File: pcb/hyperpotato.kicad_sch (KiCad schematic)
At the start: 60 parts, among them J2 Conn_01x02_Socket, J3 Conn_01x04, J4 Conn_01x04, J5 Conn_01x04, J6 Conn_01x12_Socket, J7 Conn_01x12_Socket, K1 SW_Push, K10 SW_Push, K11 SW_Push, K12 SW_Push, K13 SW_Push, K14 SW_Push, K15 SW_Push, K16 SW_Push, K17 SW_Push, K2 SW_Push, K3 SW_Push, K4 SW_Push, K5 SW_Push, K6 SW_Push, K7 SW_Push, K8 SW_Push, K9 SW_Push, SW1 SW_Push, SW2 SW_SPDT, U1 ProMicro

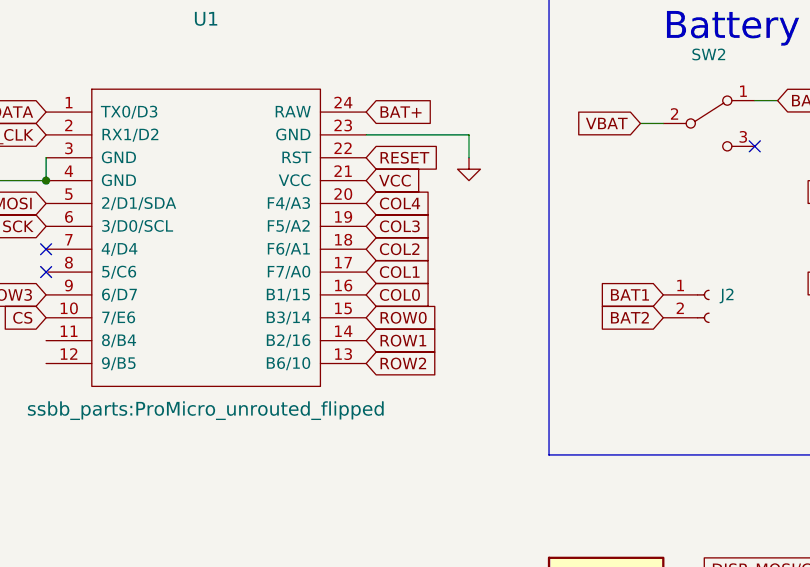
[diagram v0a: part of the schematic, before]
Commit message: Finish v2
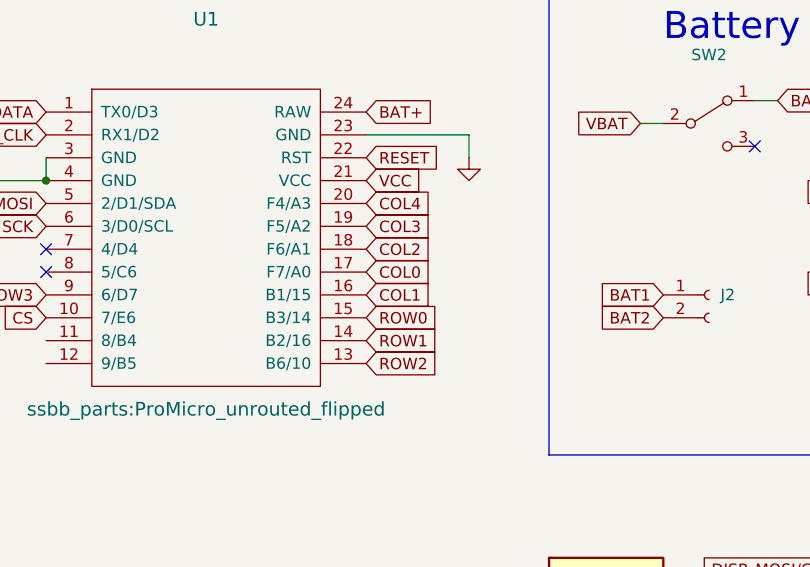
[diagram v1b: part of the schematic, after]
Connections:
- net COL0: now also U1.17 (F7/A0); no longer U1.16 (B1/15)
- net COL1: now also U1.16 (B1/15); no longer U1.17 (F7/A0)
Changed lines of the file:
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@@
     )
   )
-  (global_label "COL0" (shape input) (at 186.69 53.34 0) (fields_autoplaced)
+  (global_label "COL1" (shape input) (at 186.69 53.34 0) (fields_autoplaced)
     (effects (font (size 1.27 1.27)) (justify left))
     (property "Intersheetrefs" "${INTERSHEET_REFS}" (at 194.5133 53.34 0)
@@
     )
   )
-  (global_label "COL1" (shape input) (at 186.69 50.8 0) (fields_autoplaced)
+  (global_label "COL0" (shape input) (at 186.69 50.8 0) (fields_autoplaced)
     (effects (font (size 1.27 1.27)) (justify left))
     (property "Intersheetrefs" "${INTERSHEET_REFS}" (at 194.5133 50.8 0)

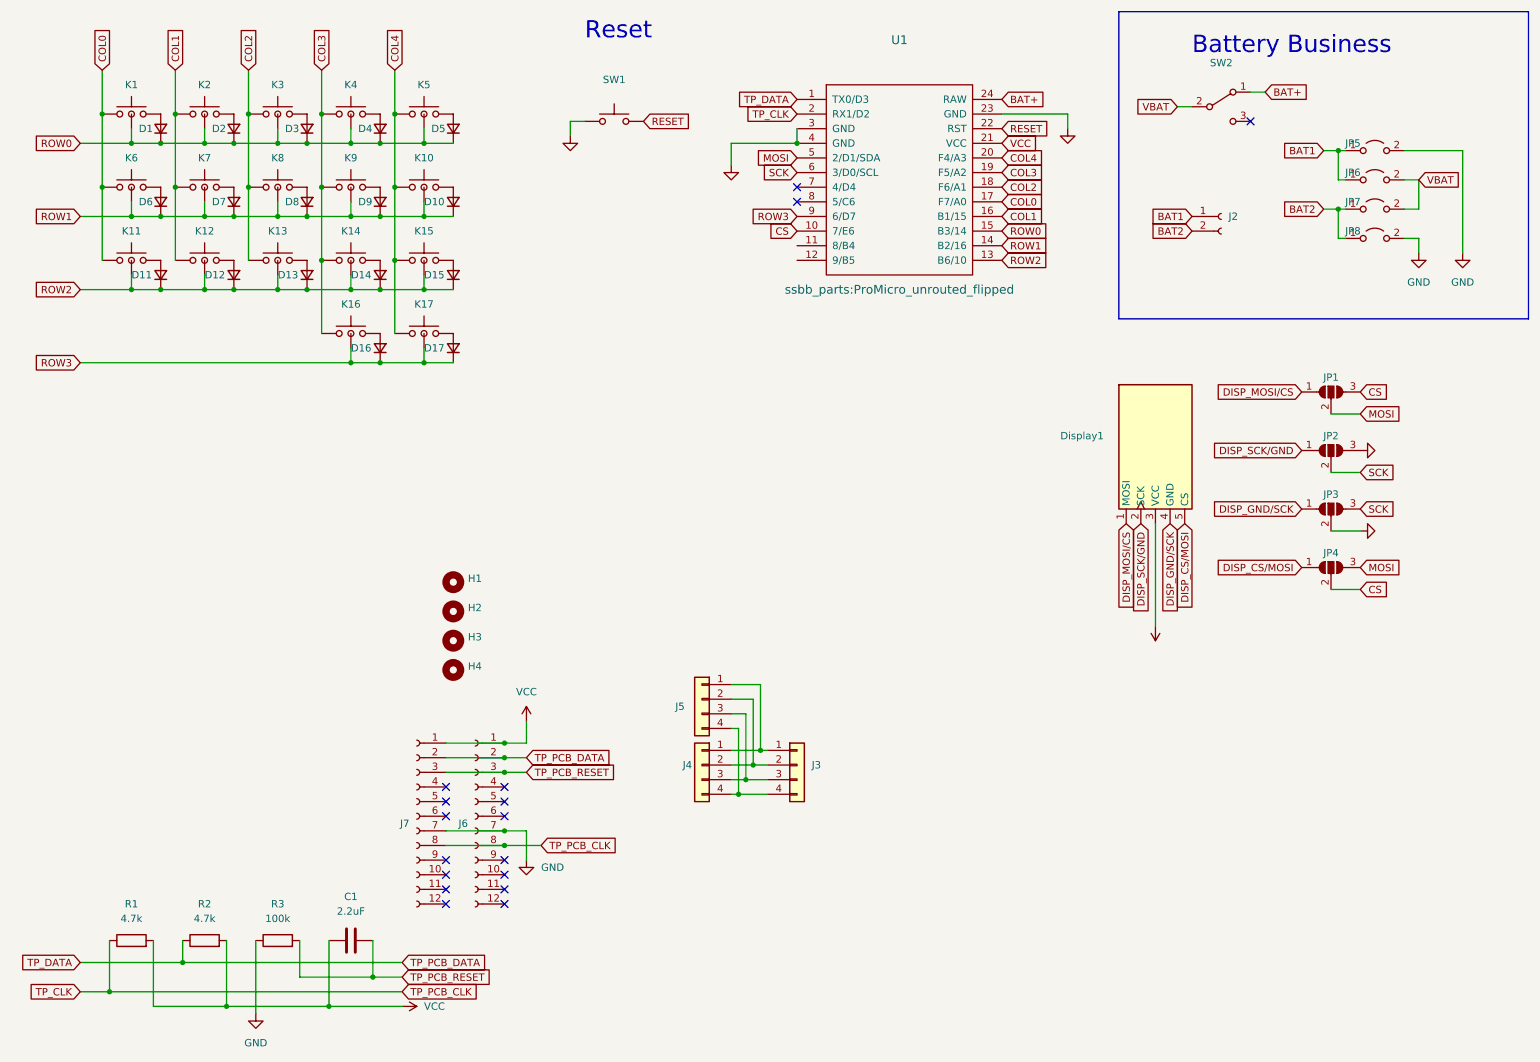
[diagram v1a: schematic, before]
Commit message: Quick and dirty tucky thumbs pcb
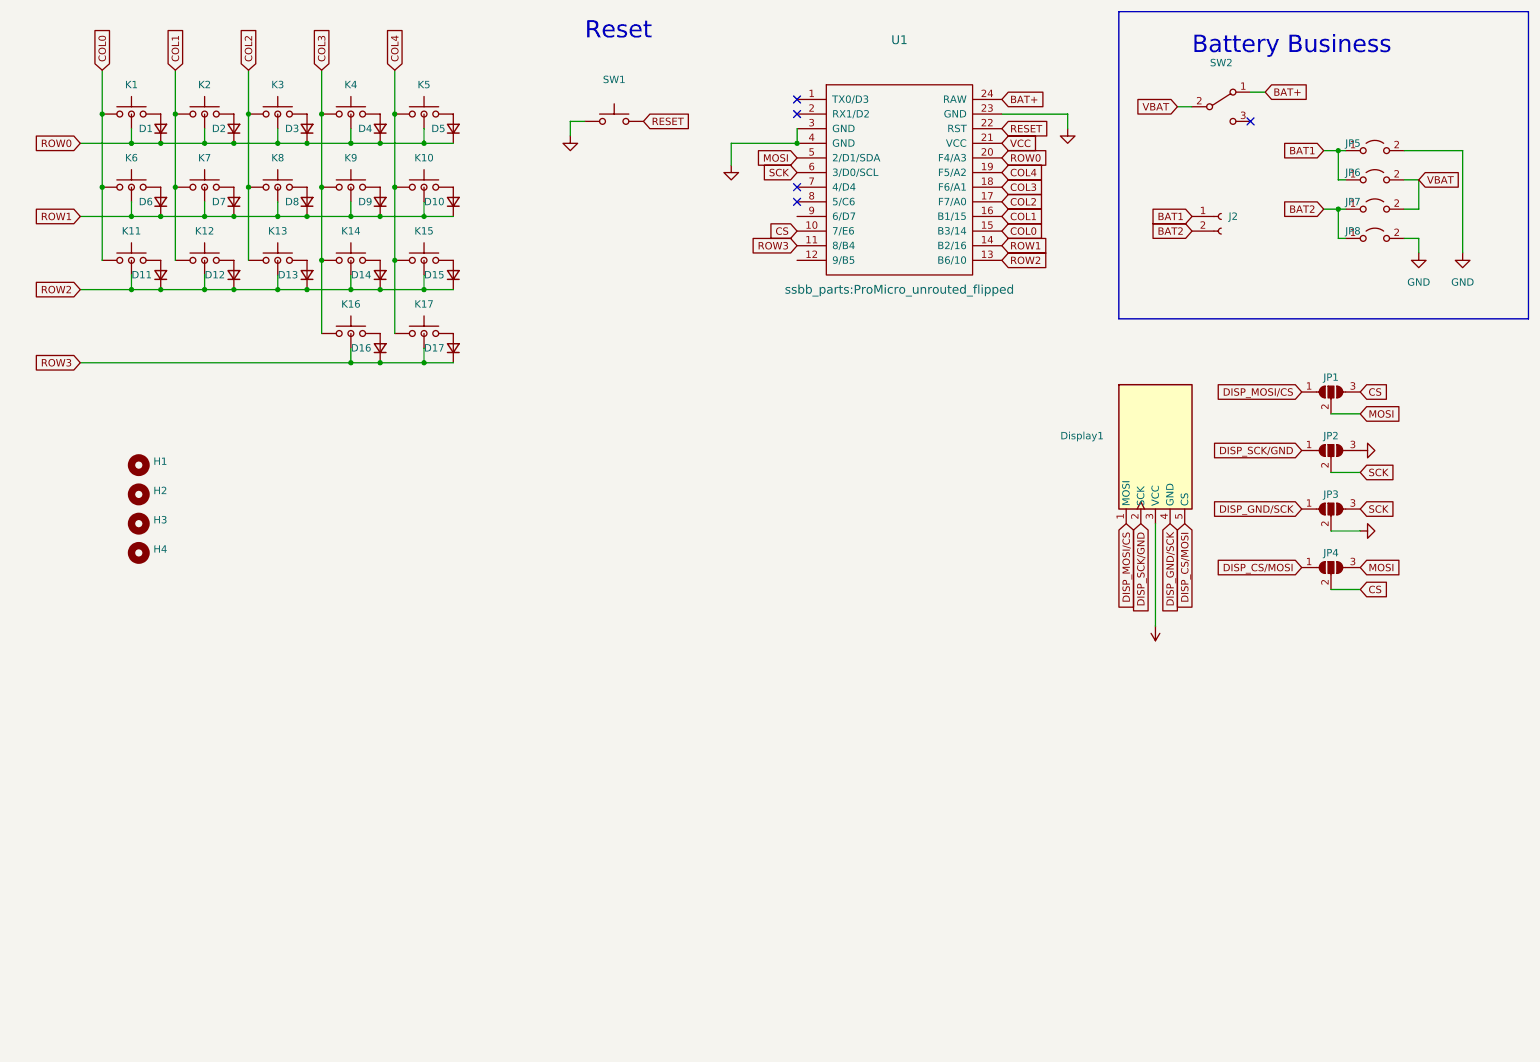
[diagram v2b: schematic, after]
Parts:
- removed C1: 2.2uF, hyperpotato:C_reversible, symbol Device:C
- removed J3: Conn_01x04, hyperpotato:Trackpoint_Connector_Reversible, symbol Connector_Generic:Conn_01x04
- removed J4, J5: Conn_01x04, hyperpotato:Trackpoint_Connector, symbol Connector_Generic:Conn_01x04
- removed J6, J7: Conn_01x12_Socket, hyperpotato:Trackpoint_PCB_Connector, symbol Connector:Conn_01x12_Socket
- removed R1, R2: 4.7k, hyperpotato:R_reversible, symbol Device:R
- removed R3: 100k, hyperpotato:R_reversible, symbol Device:R
- K1, K10, K11, K12, K13, K14, K16, K2, K3, K4, K5, K6, K7, K8, K9: footprint hyperpotato:V1_V2_HS_reversible_plated -> hyperpotato:PG1350_HS_reversible_plated
- K15: footprint hyperpotato:V1_V2_HS_reversible_plated_alt -> hyperpotato:PG1350_HS_reversible_plated
- K17: footprint hyperpotato:V1_V2_HS_reversible_plated_no_fix_pin -> hyperpotato:PG1350_HS_reversible_plated
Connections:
- net COL0: now also U1.15 (B3/14); no longer U1.17 (F7/A0)
- net COL2: now also U1.17 (F7/A0); no longer U1.18 (F6/A1)
- net COL3: now also U1.18 (F6/A1); no longer U1.19 (F5/A2)
- net COL4: now also K15.1, U1.19 (F5/A2); no longer K15.2, U1.20 (F4/A3)
- net ROW0: now also U1.20 (F4/A3); no longer U1.15 (B3/14)
- net ROW3: now also U1.11 (8/B4); no longer U1.9 (6/D7)
- net at D15.2 (A): now also K15.2; no longer K15.1
- net TP_CLK: no longer names the net of U1.2 (RX1/D2)
- net TP_DATA: no longer names the net of U1.1 (TX0/D3)
- no-connect marks 17 -> 5
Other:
- moved on the sheet: H1, H2, H3, H4

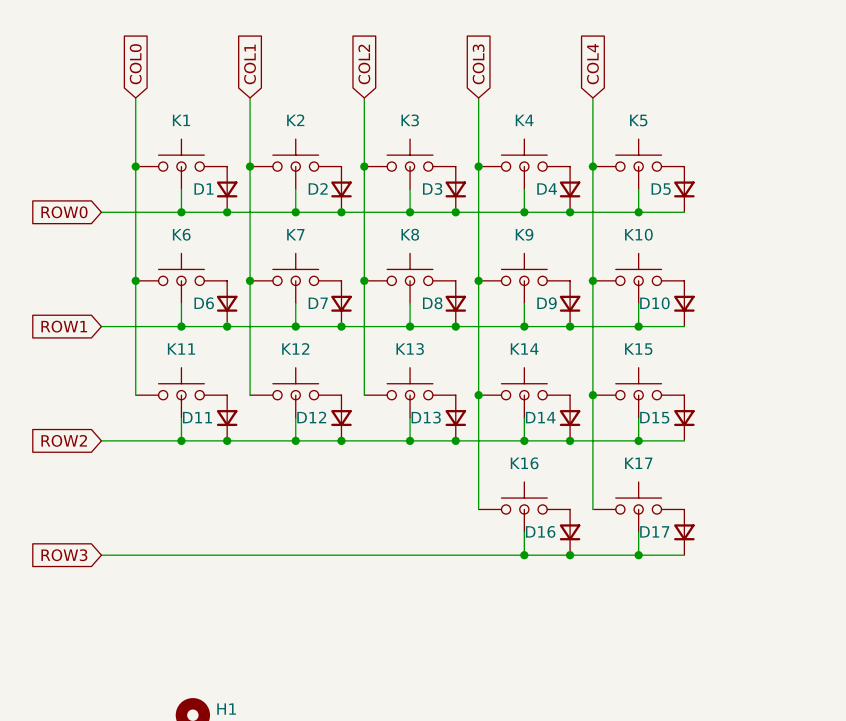
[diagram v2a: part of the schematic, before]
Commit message: Quick and dirty choc mini version
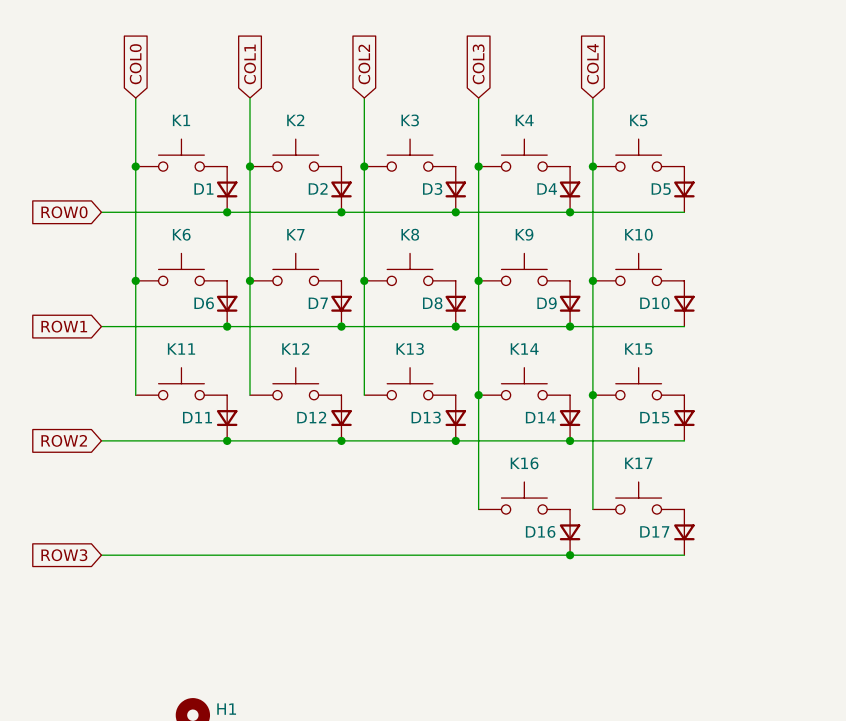
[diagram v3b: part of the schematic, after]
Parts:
- K1, K11, K6: footprint hyperpotato:PG1350_HS_reversible_plated -> hyperpotato:SW_PG1350_rev_DPB2.1; symbol hyperpotato:SW_Push -> Switch:SW_Push
- K10, K12, K13, K14, K15, K16, K17, K2, K3, K4, K5, K7, K8, K9: footprint hyperpotato:PG1350_HS_reversible_plated -> hyperpotato:Choc_Mini_PG1232_Choc_Spacing_dual_ease; symbol hyperpotato:SW_Push -> Switch:SW_Push
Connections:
- net ROW0: no longer K1.3, K2.3, K3.3, K4.3, K5.3
- net ROW1: no longer K10.3, K6.3, K7.3, K8.3, K9.3
- net ROW2: no longer K11.3, K12.3, K13.3, K14.3, K15.3
- net ROW3: no longer K16.3, K17.3
